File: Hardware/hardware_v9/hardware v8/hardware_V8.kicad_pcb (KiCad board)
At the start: 6 copper layers, 20.3 x 17 mm, 59 parts, among them IC1 TPS22960RSER, IC4 MAX-M10S-00B, IC5 LTC4065EDC#TRMPBF, IC6 W25Q128JVPIQ, J2 503548-0622, J3 USB4110-GF-A, SW4 boot, U1 STM32L432KCUx, U2 ldln025pu

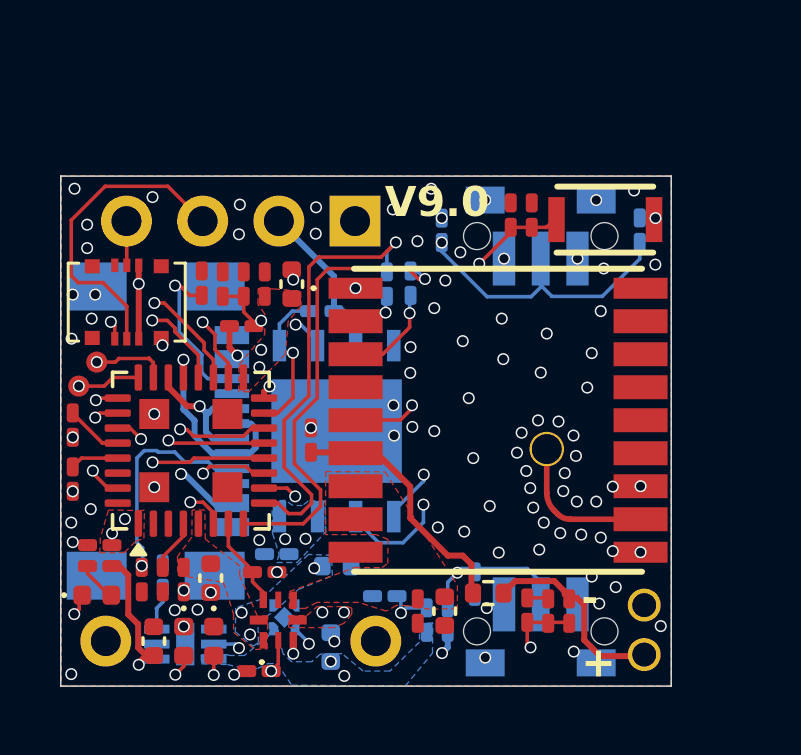
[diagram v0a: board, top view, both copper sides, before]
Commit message: up
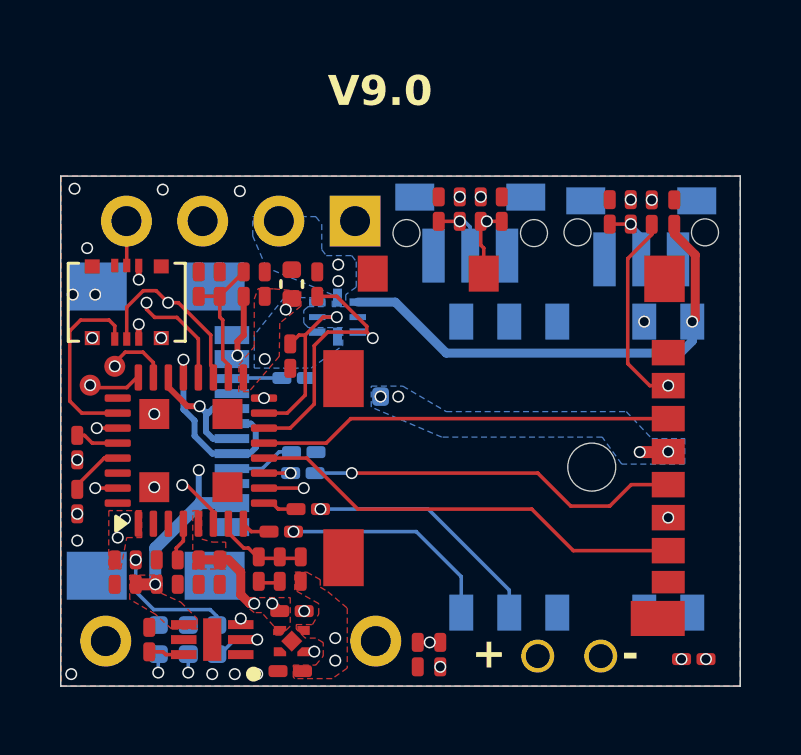
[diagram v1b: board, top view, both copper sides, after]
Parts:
- removed C18, C25, C26: 100n, Capacitor_SMD:C_0201_0603Metric_Pad0.64x0.40mm_HandSolder
- removed C28: 4.7u, Capacitor_SMD:C_0402_1005Metric
- removed IC4: MAX-M10S-00B, samacsys:MAXM10S00B
- removed IC6: W25Q128JVPIQ, samacsys2:SON127P600X500X80-9N-D
- removed R11, R12: 510R, Resistor_SMD:R_0201_0603Metric_Pad0.64x0.40mm_HandSolder
- removed R6: 20k, Resistor_SMD:R_0201_0603Metric_Pad0.64x0.40mm_HandSolder
- removed R8: 0R, Resistor_SMD:R_0402_1005Metric
- removed SW4: boot, samacsys:KXT341LHS
- removed U3: ~, samacsys2:GNSS_8mmx8mm
- added C12: 1u, Capacitor_SMD:C_0201_0603Metric_Pad0.64x0.40mm_HandSolder, F.Cu at (114.5, 92.7)
- added C21: 4.7u, Capacitor_SMD:C_0402_1005Metric, B.Cu at (104.2, 98.8)
- added J1: Micro_SD_Card_Det2, Connector_Card:microSD_HC_Molex_104031-0811, F.Cu at (108.8, 100.5)
- added PA1010D1: PA1010D, pa1010d:PA1010D, B.Cu at (106.2, 106.2)
- added R14: 470R, Resistor_SMD:R_0201_0603Metric_Pad0.64x0.40mm_HandSolder, F.Cu at (101.3, 103.3)
- added R15: 470R, Resistor_SMD:R_0201_0603Metric_Pad0.64x0.40mm_HandSolder, F.Cu at (102.2, 102.6)
- added R24: 0R, Resistor_SMD:R_0201_0603Metric_Pad0.64x0.40mm_HandSolder, F.Cu at (115.1, 107.6)
- added R25: 20k, Resistor_SMD:R_0201_0603Metric_Pad0.64x0.40mm_HandSolder, F.Cu at (108.0, 92.6)
- added R26: 22R, Resistor_SMD:R_0201_0603Metric_Pad0.64x0.40mm_HandSolder, B.Cu at (102.1, 101.4)
- C1, C4: footprint Capacitor_SMD:C_0402_1005Metric -> Capacitor_SMD:C_0201_0603Metric_Pad0.64x0.40mm_HandSolder; moved to F.Cu
- C11, C20, C7, IC5, R13, R17, R18, R5, R7, R9, U2: moved to F.Cu
- C16, C29: footprint Capacitor_SMD:C_0402_1005Metric -> Capacitor_SMD:C_0201_0603Metric_Pad0.64x0.40mm_HandSolder
- IC1, LEDBLUE1, LEDGREEN1, LEDRED1, R22, R23: moved to B.Cu
- moved R9 14.9 mm to (113.0, 92.7), turned to 90 degrees
- moved C11 13.7 mm to (108.7, 92.6), turned to 90 degrees
- moved S3 13.6 mm to (113.3, 93.5), turned to 0 degrees
- moved C20 13.2 mm to (112.3, 92.7), turned to 90 degrees
- moved R13 11.5 mm to (113.7, 92.7), turned to 90 degrees
- moved R21 10.6 mm to (101.7, 97.5), turned to 90 degrees
- moved IC1 10.3 mm to (103.2, 96.2), turned to 0 degrees
- moved R20 9.76 mm to (102.5, 95.1), turned to -90 degrees
- moved R16 9.75 mm to (100.6, 104.6), turned to 90 degrees
- moved R10 9.06 mm to (102.0, 104.6), turned to 90 degrees
- moved C8 8.36 mm to (101.3, 104.6), turned to -90 degrees
- moved R23 6.87 mm to (102.1, 100.7), turned to 0 degrees
- moved C7 6.74 mm to (106.6, 92.6)
- moved R22 4.41 mm to (101.8, 98.2), turned to 0 degrees
- moved LEDRED1 4.27 mm to (99.2, 107.0), turned to 90 degrees
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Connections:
- C11 pad 1: 3.3V_AUX -> /SD_DET
- U1 pad 10: /AUX_EN -> /SPI_CS
- U1 pad 14: /ADC_BAT -> /GPS_EN
- U1 pad 15: /SPI_CS -> /AUX_EN
- U1 pad 18: /GPS_EXTINT -> /USB_DETECT
- U1 pad 25: /B1 -> unconnected-(U1-PA15-Pad25)
- U1 pad 27: /USB_DETECT -> /SD_DET
- U1 pad 31: Net-(U1-PH3) -> /B1
- U1 pad 7: /GPS_EN -> /ADC_BAT
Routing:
- net Net-(U1-PH3): track 21.6 -> 0.00 mm, vias 2 -> 0
- net 3.3V_AUX: track 8.32 -> 29.0 mm, vias 5 -> 10
- net /SD_DET: track 0.00 -> 19.7 mm, vias 0 -> 2
- net /ADC_BAT: track 22.4 -> 3.09 mm, vias 2 -> 0
- net /SPI_CS: track 5.13 -> 21.5 mm, vias 1 -> 2
- net 3.3V_GPS: track 0.00 -> 16.2 mm, vias 0 -> 1
- net GND: track 15.0 -> 0.00 mm, vias 94 -> 18
- net /GPS_RX: track 15.5 -> 0.96 mm, vias 1 -> 0
- net BAT+: track 6.72 -> 20.6 mm, vias 2 -> 5
- net /GPS_TX: track 14.8 -> 1.15 mm, vias 1 -> 0
- net /GPS_EXTINT: track 12.9 -> 0.00 mm, vias 2 -> 0
- net Net-(J1-CLK): track 0.00 -> 12.5 mm, vias 0 -> 1
- net /SPI_CLK: track 13.8 -> 1.40 mm, vias 2 -> 1
- net Net-(PA1010D1-VBACKUP): track 0.00 -> 12.1 mm, vias 0 -> 2
- net /OLED_SCL: track 19.1 -> 9.34 mm
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- added copper zone on F.Cu, net BAT+
- added copper zone on F.Cu, net vusb
- removed copper zone on In3.Cu, net +3.3V
- removed copper zone on F.Cu, net 3.3V_AUX
- removed copper zone on In3.Cu, net 3.3V_AUX
- removed copper zone on F.Cu, net 3.3V_GPS
- removed copper zone on B.Cu, net BAT+
- removed copper zone on In3.Cu, net BAT+
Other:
- board size 20.3 x 17 mm -> 22.7 x 17 mm

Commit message: up
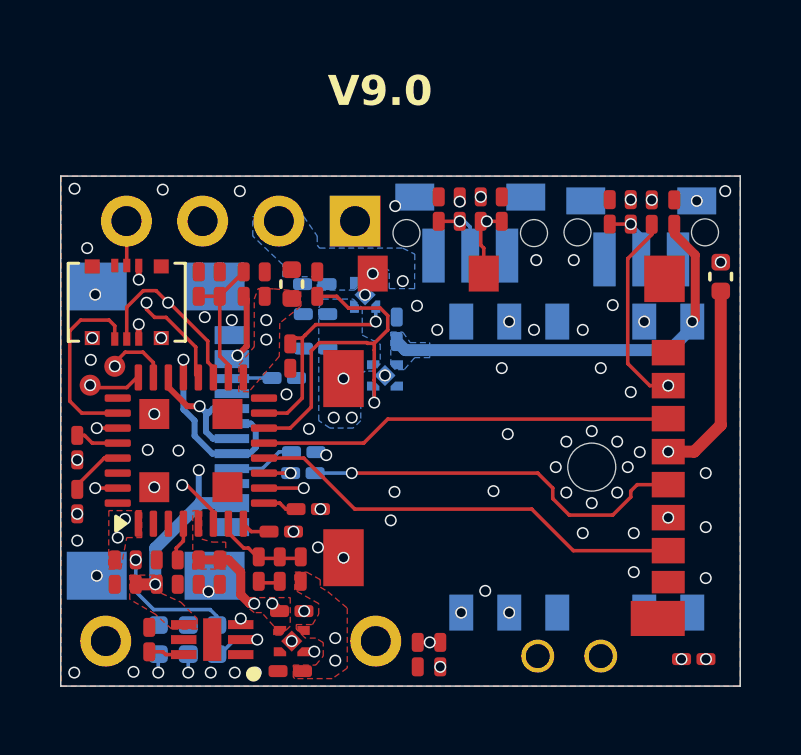
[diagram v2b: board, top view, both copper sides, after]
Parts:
- removed IC1: TPS22960RSER, samacsys2:TPS22960RSER
- removed R20: 100k, Resistor_SMD:R_0201_0603Metric_Pad0.64x0.40mm_HandSolder
- added C2: 1u, Capacitor_SMD:C_0201_0603Metric_Pad0.64x0.40mm_HandSolder, F.Cu at (101.7, 106.0)
- added C3: 1u, Capacitor_SMD:C_0201_0603Metric_Pad0.64x0.40mm_HandSolder, B.Cu at (102.5, 96.1)
- added C5: 1u, Capacitor_SMD:C_0201_0603Metric_Pad0.64x0.40mm_HandSolder, B.Cu at (105.2, 96.6)
- added C6: 1u, Capacitor_SMD:C_0201_0603Metric_Pad0.64x0.40mm_HandSolder, B.Cu at (102.5, 97.2)
- added R27: 100k, Resistor_SMD:R_0201_0603Metric_Pad0.64x0.40mm_HandSolder, F.Cu at (102.5, 95.1)
- added U3: ldln025pu, samacsys:ldln025pu, B.Cu at (104.8, 98.1)
- added U5: ldln025pu, samacsys:ldln025pu, B.Cu at (104.1, 95.5)
- C1: moved to B.Cu
- C21: moved to F.Cu
- moved C21 12.5 mm to (116.0, 94.8), turned to 90 degrees
- moved C1 10.9 mm to (102.5, 95.1), turned to 180 degrees
- moved R22 0.33 mm to (101.5, 98.2)
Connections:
- C1 pad 1: +3.3V -> 3.3V_AUX
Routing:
- net BAT+: track 20.6 -> 0.00 mm, vias 5 -> 7
- net +3.3V: track 38.3 -> 17.9 mm
- net 3.3V_AUX: track 29.0 -> 21.0 mm, vias 10 -> 7
- net vusb: track 13.1 -> 8.75 mm
- net /GPS_EN: track 9.16 -> 12.4 mm
- net 3.3V_GPS: track 16.2 -> 14.1 mm
- net /AUX_EN: track 6.19 -> 7.14 mm
- net Net-(PA1010D1-VBACKUP): track 12.1 -> 13.0 mm
- net /B_PW: track 22.4 -> 23.3 mm
- net Net-(J1-CLK): track 12.5 -> 13.1 mm
- net Net-(PA1010D1-TX): vias 1 -> 2
- net Net-(PA1010D1-RX): vias 1 -> 2
- net GND: vias 18 -> 68
- added copper zone on In3.Cu, net +3.3V
- added copper zone on In3.Cu, net 3.3V_AUX
- added copper zone on B.Cu, net 3.3V_GPS
- added copper zone on B.Cu, net BAT+
- added copper zone on In3.Cu, net BAT+
- added copper zone on In2.Cu, net GND
- added copper zone on In3.Cu, net GND
- added copper zone on In3.Cu, net vusb
- removed copper zone on B.Cu, net +3.3V
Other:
- board text removed: "+"
- board text removed: "-"
